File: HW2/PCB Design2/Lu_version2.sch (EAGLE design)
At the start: 22 parts, among them J2 USB-MB-H

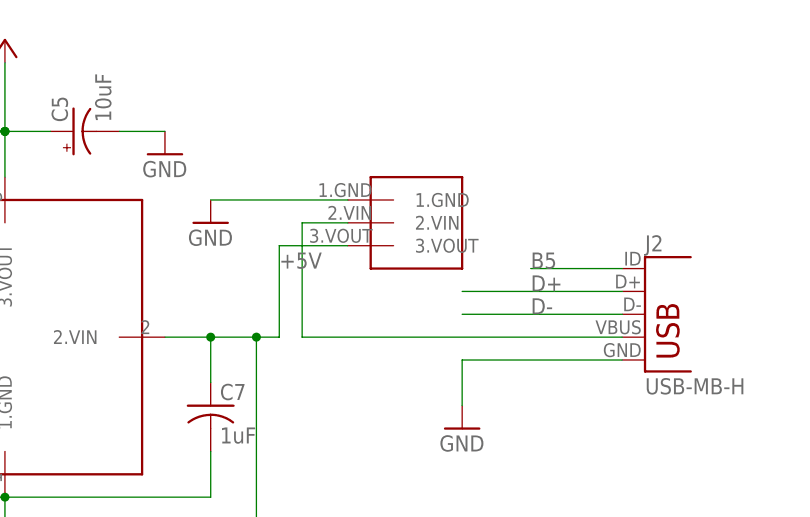
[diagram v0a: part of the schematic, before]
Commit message: edit
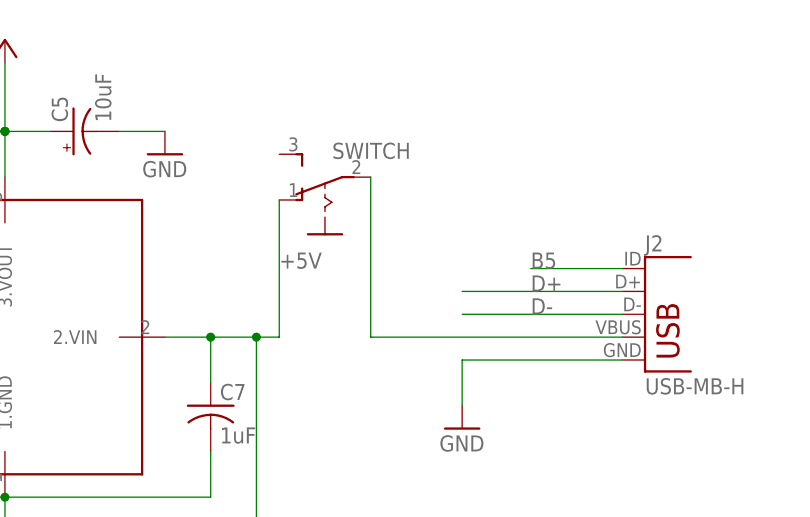
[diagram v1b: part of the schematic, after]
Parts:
- removed U$3: (no value), Lu_hw2:SWITCH
- added SWITCH: (no value), Lu_hw2:255SB
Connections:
- net +5V: now also SWITCH.O; no longer U$3.3.VOUT
- net GND: no longer U$3.1.GND
- net N$1: now also SWITCH.P; no longer U$3.2.VIN
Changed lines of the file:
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@@
 <part name="+3V4" library="Lu_hw2" deviceset="+3V3" device=""/>
 <part name="P+1" library="Lu_hw2" deviceset="+5V" device=""/>
-<part name="GND8" library="Lu_hw2" deviceset="GND" device=""/>
 <part name="LED2" library="Lu_hw2" deviceset="LED" device="3MM"/>
 <part name="GND16" library="Lu_hw2" deviceset="GND" device=""/>
@@
 <part name="R2" library="Lu_hw2" deviceset="R-US_" device="0207/10" value="10K"/>
 <part name="+3V6" library="Lu_hw2" deviceset="+3V3" device=""/>
-<part name="U$3" library="Lu_hw2" deviceset="SWITCH" device=""/>
+<part name="SWITCH" library="Lu_hw2" deviceset="255SB" device=""/>
 </parts>
 <sheets>
@@
 </instance>
 <instance part="P+1" gate="1" x="43.18" y="58.42" rot="R270"/>
-<instance part="GND8" gate="1" x="-25.4" y="149.86"/>
 <instance part="LED2" gate="G$1" x="58.42" y="91.44" rot="R90"/>
 <instance part="GND16" gate="1" x="73.66" y="88.9"/>
@@
 </instance>
 <instance part="+3V6" gate="G$1" x="71.12" y="99.06" rot="R270"/>
-<instance part="U$3" gate="G$1" x="-5.08" y="154.94"/>
+<instance part="SWITCH" gate="1" x="-12.7" y="152.4" smashed="yes" rot="R90">
+<attribute name="NAME" x="-3.175" y="158.75" size="1.778" layer="95" rot="R180"/>
+<attribute name="VALUE" x="-15.875" y="148.59" size="1.778" layer="96" rot="R180"/>
+</instance>
 </instances>
 <busses>
@@
 <pinref part="GND10" gate="1" pin="GND"/>
 <wire x1="17.78" y1="55.88" x2="43.18" y2="55.88" width="0.1524" layer="91"/>
-</segment>
-<segment>
-<wire x1="-10.16" y1="152.4" x2="-25.4" y2="152.4" width="0.1524" layer="91"/>
-<pinref part="GND8" gate="1" pin="GND"/>
-<pinref part="U$3" gate="G$1" pin="1.GND"/>
 </segment>
 <segment>
@@
 <wire x1="-17.78" y1="137.16" x2="-20.32" y2="137.16" width="0.1524" layer="91"/>
 <junction x="-20.32" y="137.16"/>
-<wire x1="-10.16" y1="147.32" x2="-17.78" y2="147.32" width="0.1524" layer="91"/>
-<wire x1="-17.78" y1="147.32" x2="-17.78" y2="137.16" width="0.1524" layer="91"/>
+<wire x1="-17.78" y1="152.4" x2="-17.78" y2="137.16" width="0.1524" layer="91"/>
 <label x="-17.78" y="144.78" size="1.778" layer="95"/>
-<pinref part="U$3" gate="G$1" pin="3.VOUT"/>
+<pinref part="SWITCH" gate="1" pin="O"/>
 </segment>
 </net>
@@
 <segment>
 <pinref part="J2" gate="G$1" pin="VBUS"/>
-<wire x1="20.32" y1="137.16" x2="-15.24" y2="137.16" width="0.1524" layer="91"/>
-<wire x1="-15.24" y1="137.16" x2="-15.24" y2="149.86" width="0.1524" layer="91"/>
-<wire x1="-15.24" y1="149.86" x2="-10.16" y2="149.86" width="0.1524" layer="91"/>
-<pinref part="U$3" gate="G$1" pin="2.VIN"/>
-</segment>
-</net>
+<wire x1="20.32" y1="137.16" x2="-7.62" y2="137.16" width="0.1524" layer="91"/>
+<wire x1="-7.62" y1="137.16" x2="-7.62" y2="154.94" width="0.1524" layer="91"/>
+<pinref part="SWITCH" gate="1" pin="P"/>
+</segment>
+</net>
